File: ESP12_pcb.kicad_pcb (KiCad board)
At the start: 2 copper layers, 36.8 x 36.8 mm, 32 parts, among them CON1 ZX62D1-B-5PA(30), J1 CONN_01X02, J2 CONN_01X02_FEMALE, Q1 IRLML9301TRPBF, Q2 IRLML9301TRPBF, U1 LD1117DT33TR, U2 TPS61090

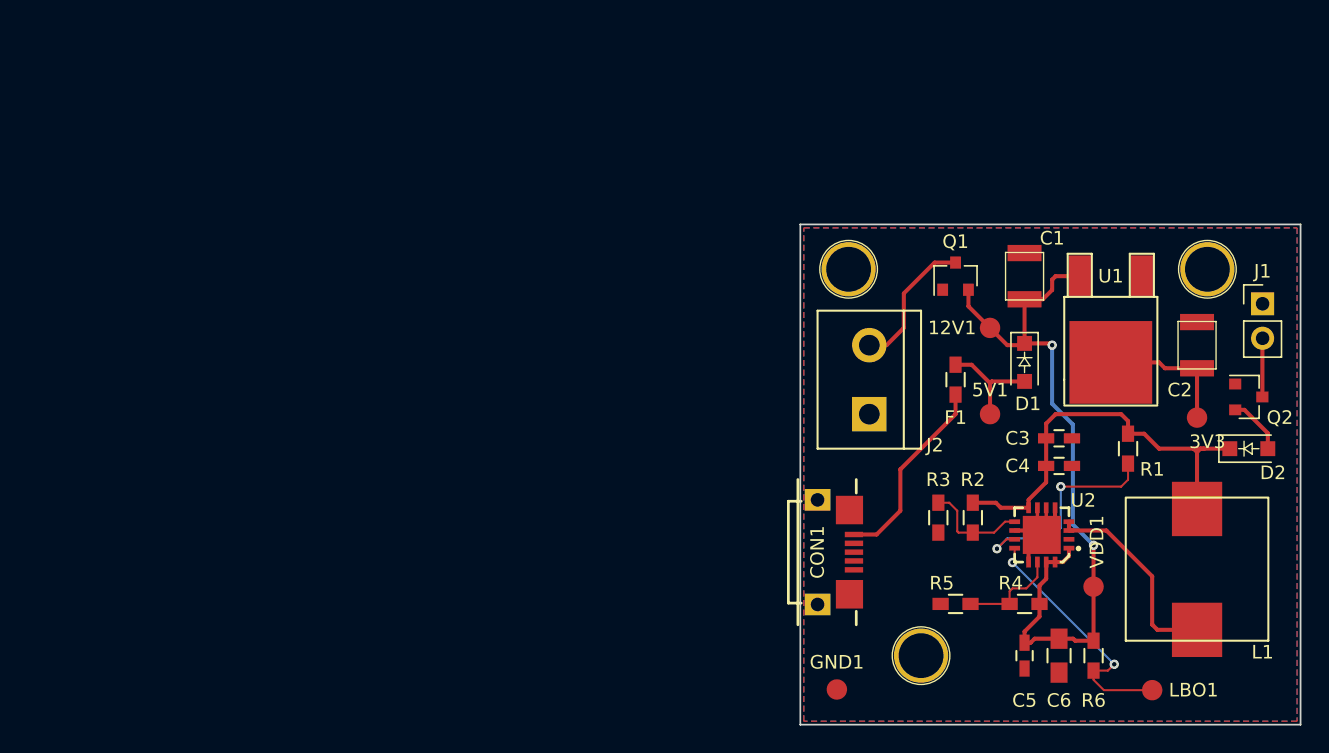
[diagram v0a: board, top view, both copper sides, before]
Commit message: Version V0.1 sended to fabrication
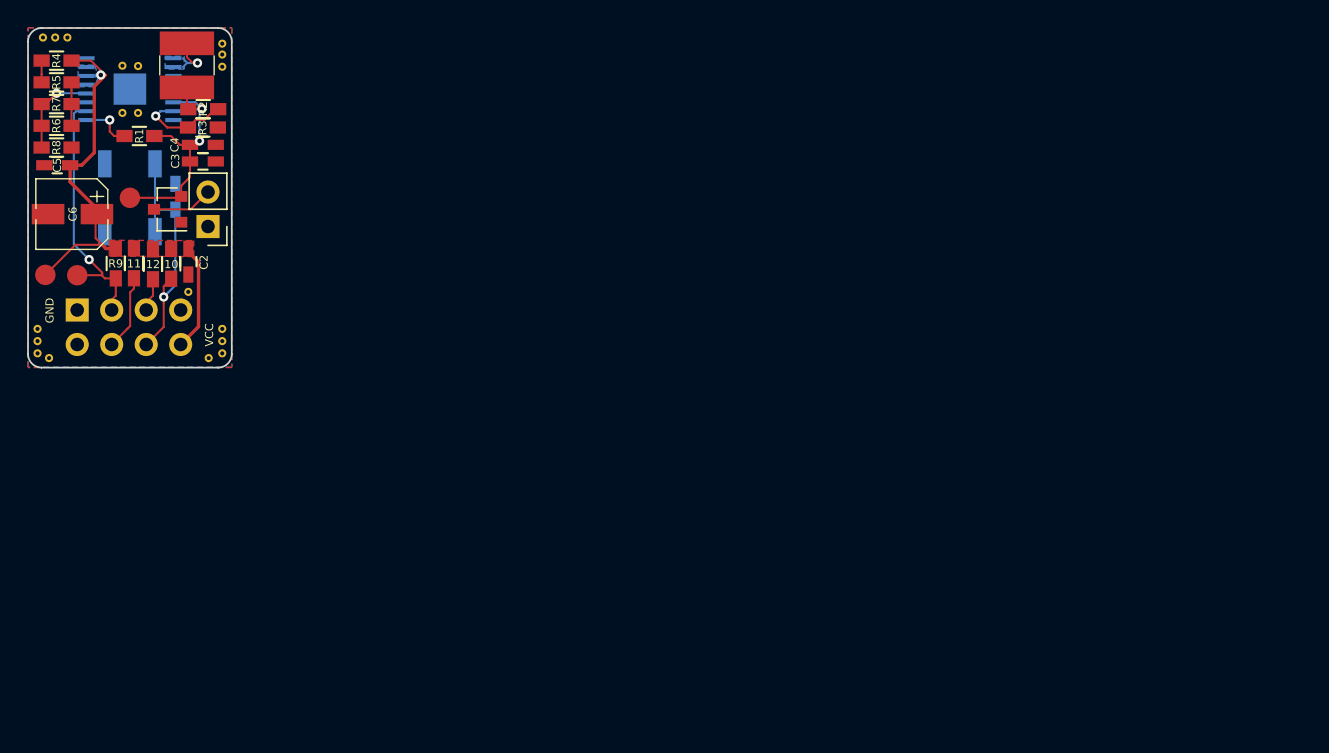
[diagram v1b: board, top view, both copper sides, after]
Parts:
- removed 12V1, 3V3, 5V1, GND1, LBO1, VDD1: TEST, Measurement_Points:Measurement_Point_Round-SMD-Pad_Small
- removed CON1: ZX62D1-B-5PA(30), papayagroup:USB-micro-B_Hirose
- removed D1, D2: MBR120VLSFT3G, Diodes_SMD:D_SOD-123F
- removed F1: 0603L100SLYR, Resistors_SMD:R_0603_HandSoldering
- removed J2: CONN_01X02_FEMALE, Connectors:bornier2
- removed Q1: IRLML9301TRPBF, TO_SOT_Packages_SMD:SOT-23
- removed the REF** at (108.0, 111.8)
- removed the REF** at (129.0, 83.3)
- removed the REF** at (102.6, 83.3)
- removed U2: TPS61090, papayagroup:QFN65P400X400X100-17N
- added J3: Conn_02x04_Odd_Even, Pin_Headers:Pin_Header_Straight_2x04_Pitch2.54mm, B.Cu at (45.8, 86.3)
- added R10: 10k, Resistors_SMD:R_0603_HandSoldering, F.Cu at (52.7, 82.9)
- added R11: 10k, Resistors_SMD:R_0603_HandSoldering, F.Cu at (50.0, 82.9)
- added R12: 10k, Resistors_SMD:R_0603_HandSoldering, F.Cu at (51.4, 83.0)
- added R7: 0, Resistors_SMD:R_0603_HandSoldering, F.Cu at (44.3, 71.2)
- added R8: 220k, Resistors_SMD:R_0603_HandSoldering, F.Cu at (44.3, 74.3)
- added R9: 1M, Resistors_SMD:R_0603_HandSoldering, F.Cu at (48.7, 82.9)
- added REF**: via0305, papayagroup:via0305, F.Cu at (42.9, 87.7)
- added REF**: via0305, papayagroup:via0305, F.Cu at (43.3, 66.2)
- added REF**: via0305, papayagroup:via0305, F.Cu at (44.2, 66.2)
- added REF**: via0305, papayagroup:via0305, F.Cu at (56.5, 66.7)
- added REF**: via0305, papayagroup:via0305, F.Cu at (56.5, 67.5)
- added REF**: via0305, papayagroup:via0305, F.Cu at (56.5, 68.4)
- added REF**: via0305, papayagroup:via0305, F.Cu at (50.3, 71.8)
- added REF**: via0305, papayagroup:via0305, F.Cu at (49.1, 71.8)
- added REF**: via0305, papayagroup:via0305, F.Cu at (50.3, 68.3)
- added REF**: via0305, papayagroup:via0305, F.Cu at (49.1, 68.3)
- added REF**: via0305, papayagroup:via0305, F.Cu at (54.0, 85.0)
- added REF**: via0305, papayagroup:via0305, F.Cu at (56.5, 87.7)
- added REF**: via0305, papayagroup:via0305, F.Cu at (56.5, 88.6)
- added REF**: via0305, papayagroup:via0305, F.Cu at (56.5, 89.5)
- added REF**: via0305, papayagroup:via0305, F.Cu at (55.5, 89.8)
- added REF**: via0305, papayagroup:via0305, F.Cu at (43.8, 89.8)
- added REF**: via0305, papayagroup:via0305, F.Cu at (42.9, 88.6)
- added REF**: via0305, papayagroup:via0305, F.Cu at (42.9, 89.5)
- added REF**: via0305, papayagroup:via0305, F.Cu at (45.1, 66.2)
- added SW1: SW_Push, papayagroup:button_4pin, B.Cu at (49.7, 78.0)
- added TP1: bat, Measurement_Points:Measurement_Point_Round-SMD-Pad_Small, F.Cu at (49.7, 78.0)
- added TP2: vdd, Measurement_Points:Measurement_Point_Round-SMD-Pad_Small, F.Cu at (43.5, 83.7)
- added TP3: LBO, Measurement_Points:Measurement_Point_Round-SMD-Pad_Small, F.Cu at (45.8, 83.8)
- C1: footprint papayagroup:C_3528 -> Capacitors_SMD:C_0603_HandSoldering; moved to B.Cu
- C2: value 10uF -> 100nF; footprint papayagroup:C_3528 -> Capacitors_SMD:C_0603_HandSoldering
- C6: footprint Capacitors_SMD:C_0805_HandSoldering -> papayagroup:smd_5_5.4
- L1: footprint papayagroup:L_bourns -> papayagroup:smd_L_4532
- R4: value 1,87M -> 2M
- R5: value 200k -> 2M
- R6: value 1M -> 12M
- U1: value LD1117DT33TR -> TPS61030PWR; footprint TO_SOT_Packages_SMD:TO-252-2Lead -> papayagroup:R-PDSO-16; moved to B.Cu
- moved R6 85.7 mm to (44.3, 72.8), turned to 180 degrees
- moved L1 83.1 mm to (53.9, 68.3), turned to 180 degrees
- moved R4 81.7 mm to (44.3, 68.0)
- moved Q2 80.8 mm to (52.5, 78.9), turned to 180 degrees
- moved C5 79.9 mm to (44.4, 75.7), turned to 180 degrees
- moved C6 79.6 mm to (45.5, 79.2)
- moved J1 77.9 mm to (55.5, 80.2), turned to 180 degrees
- moved R5 76.5 mm to (44.3, 69.5), turned to 0 degrees
- moved R1 76.3 mm to (50.4, 73.5), turned to 180 degrees
- moved C2 74.5 mm to (54.0, 82.8)
- moved U1 73.5 mm to (49.7, 70.0), turned to 270 degrees
- moved C4 67.3 mm to (55.1, 74.2)
- moved C3 66.2 mm to (55.1, 75.4)
- moved R2 64.1 mm to (55.1, 71.5), turned to 0 degrees
- moved C1 62.8 mm to (53.0, 78.0), turned to 90 degrees
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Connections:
- C1 pad 1: VDD -> /RST
- C2 pad 1: +3V3 -> VDD
- C3 pad 1: Net-(C3-Pad1) -> +BATT
- C4 pad 1: Net-(C3-Pad1) -> +BATT
- L1 pad 1: Net-(C3-Pad1) -> +BATT
- R1 pad 1: Net-(C3-Pad1) -> +BATT
- R2 pad 1: Net-(C3-Pad1) -> +BATT
- R5 pad 2: GND -> Net-(R5-Pad2)
- R6 pad 1: VDD -> Net-(R5-Pad2)
- R6 pad 2: /LBO -> /FB
- U1 pad 1: GND -> Net-(L1-Pad2)
- U1 pad 2: +3V3 -> Net-(L1-Pad2)
- U1 pad 3: VDD -> GND
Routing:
- net Net-(C3-Pad1): track 31.8 -> 0.00 mm
- net /RST: track 0.00 -> 19.6 mm, vias 0 -> 1
- net VDD: track 50.0 -> 32.9 mm, vias 2 -> 1
- net +BATT: track 4.25 -> 19.5 mm, vias 0 -> 2
- net Net-(CON1-Pad1): track 14.4 -> 0.00 mm
- net GND: track 13.7 -> 0.00 mm
- net /TPEN: track 16.3 -> 3.79 mm, vias 2 -> 1
- net Net-(L1-Pad2): track 15.2 -> 4.41 mm, vias 0 -> 1
- net Net-(J2-Pad2): track 10.4 -> 0.00 mm
- net +3V3: track 10.2 -> 0.00 mm
- net +5V: track 7.98 -> 0.00 mm
- net /FB: track 0.00 -> 6.29 mm, vias 0 -> 1
- net Net-(R4-Pad2): track 7.40 -> 1.60 mm
- net /CH_PD: track 0.00 -> 5.55 mm
- net +12V: track 5.26 -> 0.00 mm
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- added copper zone on B.Cu, net Net-(L1-Pad2)
- added copper zone on B.Cu, net VDD
- added copper zone on F.Cu, net VDD
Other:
- board size 36.8 x 36.8 mm -> 15 x 25 mm
- board text added: "10"
- board text added: "11"
- board text added: "12"
- board text added: "C1"
- board text added: "C2"
- board text added: "C3"
- board text added: "C4"
- board text added: "C5"
- board text added: "C6"
- board text added: "GND"
- board text added: "IoT Button V0.1 Darkomen"
- board text added: "R1"
- board text added: "R2"
- board text added: "R3"
- board text added: "R4"
- board text added: "R5"
- board text added: "R6"
- board text added: "R7"
- board text added: "R8"
- board text added: "R9"
- board text added: "VCC"
